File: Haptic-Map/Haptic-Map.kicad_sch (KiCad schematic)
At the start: 5 parts, among them U1 ESP32-S3-MINI-1, U2 AMS1117-3.3

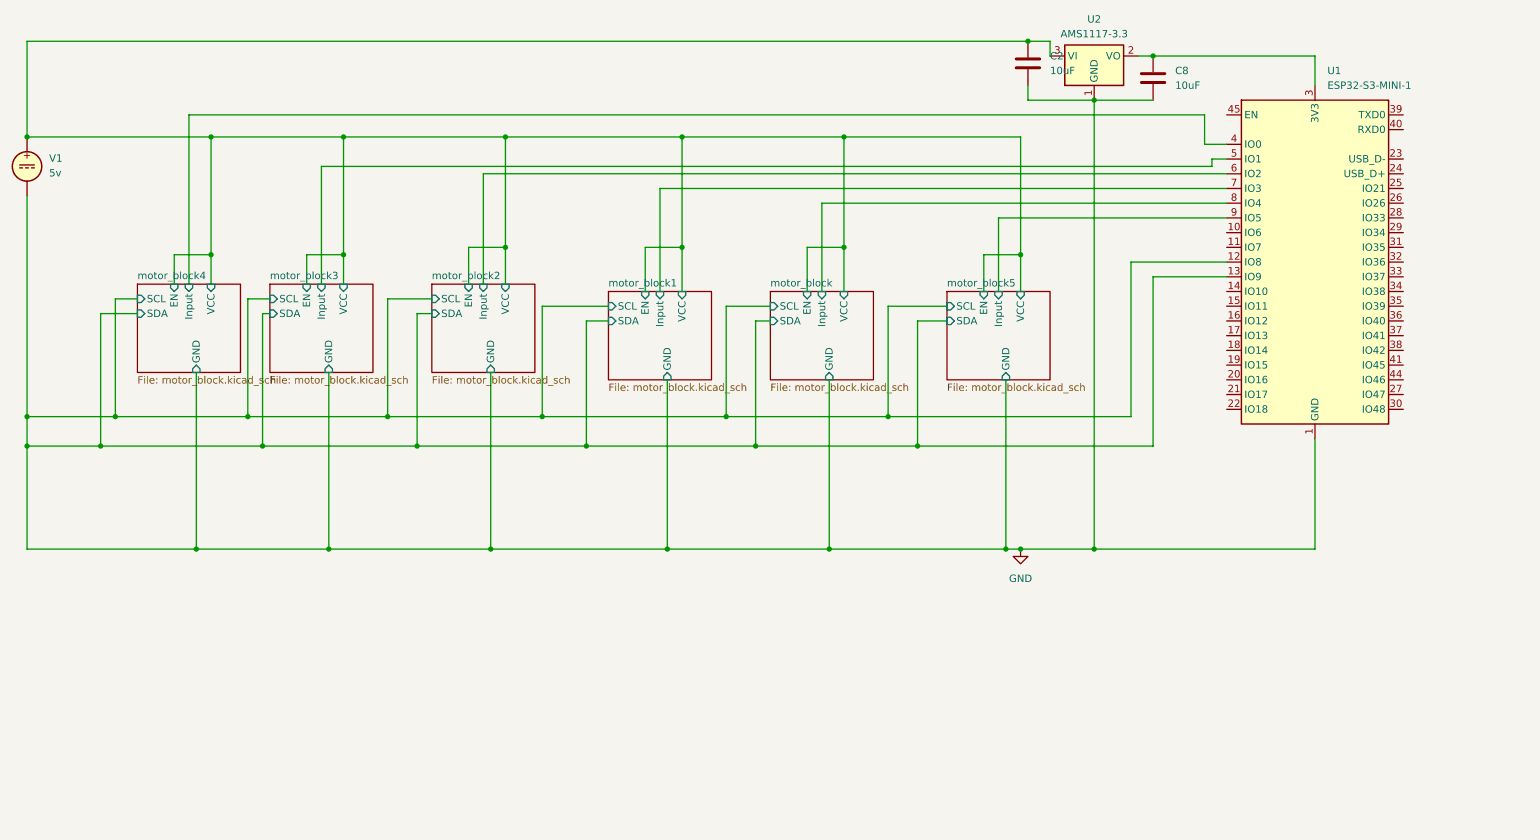
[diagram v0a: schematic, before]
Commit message: i like watching I2C rail my circuit
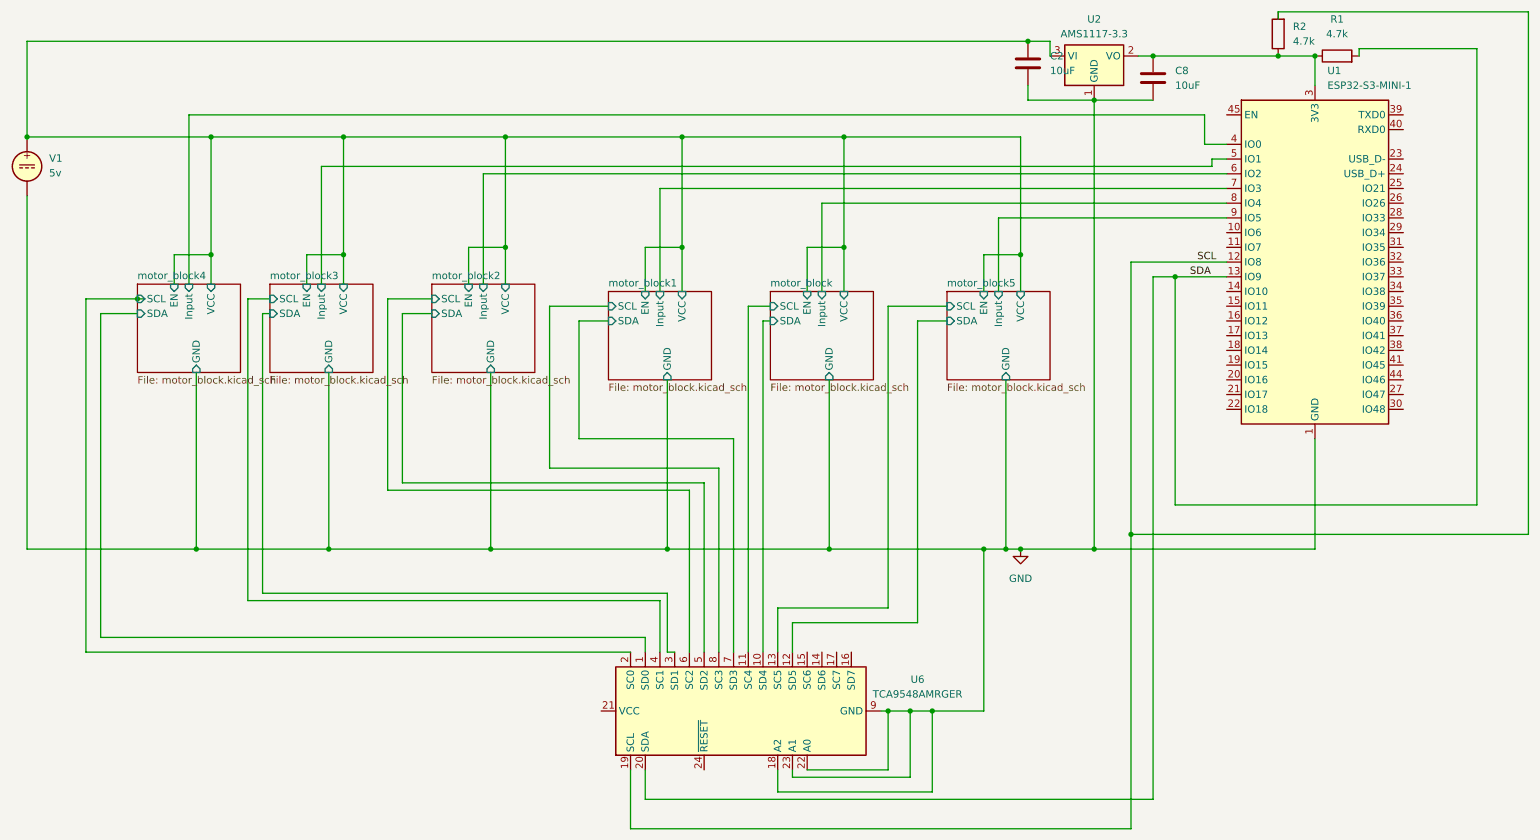
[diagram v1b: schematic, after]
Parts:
- added R1, R2: 4.7k, symbol Device:R
- added U6: TCA9548AMRGER, Package_DFN_QFN:Texas_RGE0024C_VQFN-24-1EP_4x4mm_P0.5mm_EP2.1x2.1mm, symbol Interface_Expansion:TCA9548AMRGER
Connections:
- net GND: now also U6.18 (A2), U6.22 (A0), U6.23 (A1), U6.9 (GND); no longer U1.12 (IO8), U1.13 (IO9)
- net at C8.1, U1.3 (3V3), U2.2 (VO): now also R1.1, R2.1
- new net SCL: R2.2, U1.12 (IO8), U6.19 (SCL)
- new net SDA: R1.2, U1.13 (IO9), U6.20 (SDA)
- new net motor_block/SCL: U6.11 (SC4)
- new net motor_block/SDA: U6.10 (SD4)
- new net motor_block1/SCL: U6.8 (SC3)
- new net motor_block1/SDA: U6.7 (SD3)
- new net motor_block2/SCL: U6.6 (SC2)
- new net motor_block2/SDA: U6.5 (SD2)
- new net motor_block3/SCL: U6.4 (SC1)
- new net motor_block3/SDA: U6.3 (SD1)
- new net motor_block4/SCL: U6.2 (SC0)
- new net motor_block4/SDA: U6.1 (SD0)
- new net motor_block5/SCL: U6.13 (SC5)
- new net motor_block5/SDA: U6.12 (SD5)
